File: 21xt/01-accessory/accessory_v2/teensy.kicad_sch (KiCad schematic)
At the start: 20 parts, among them Q3 BSS138, U1 DEV-16771, U2 TPS22915BYFPR

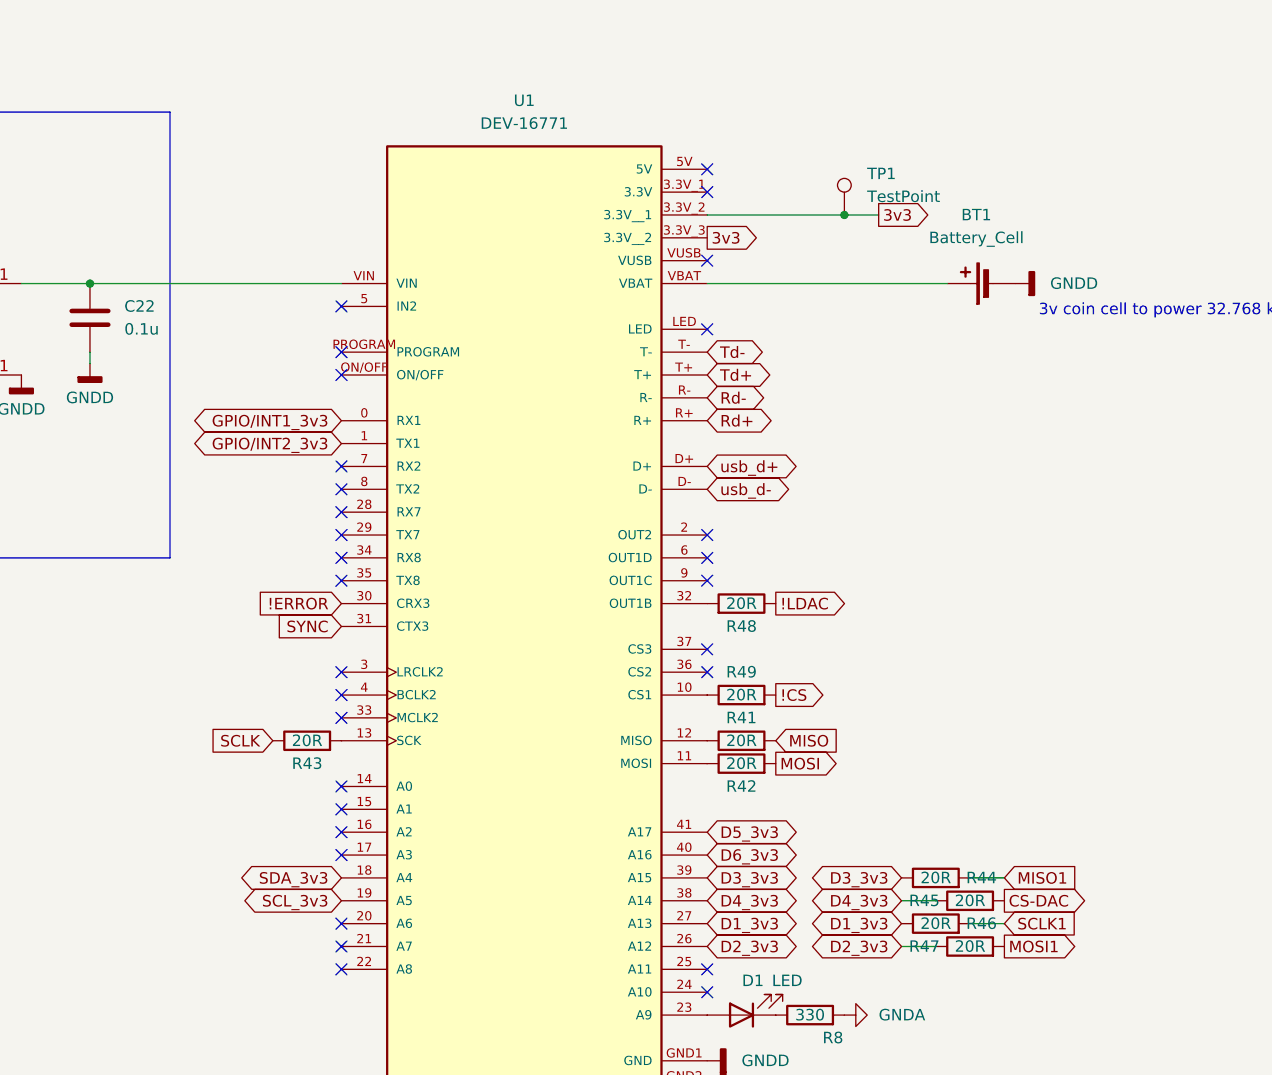
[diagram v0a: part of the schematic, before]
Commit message: laied out
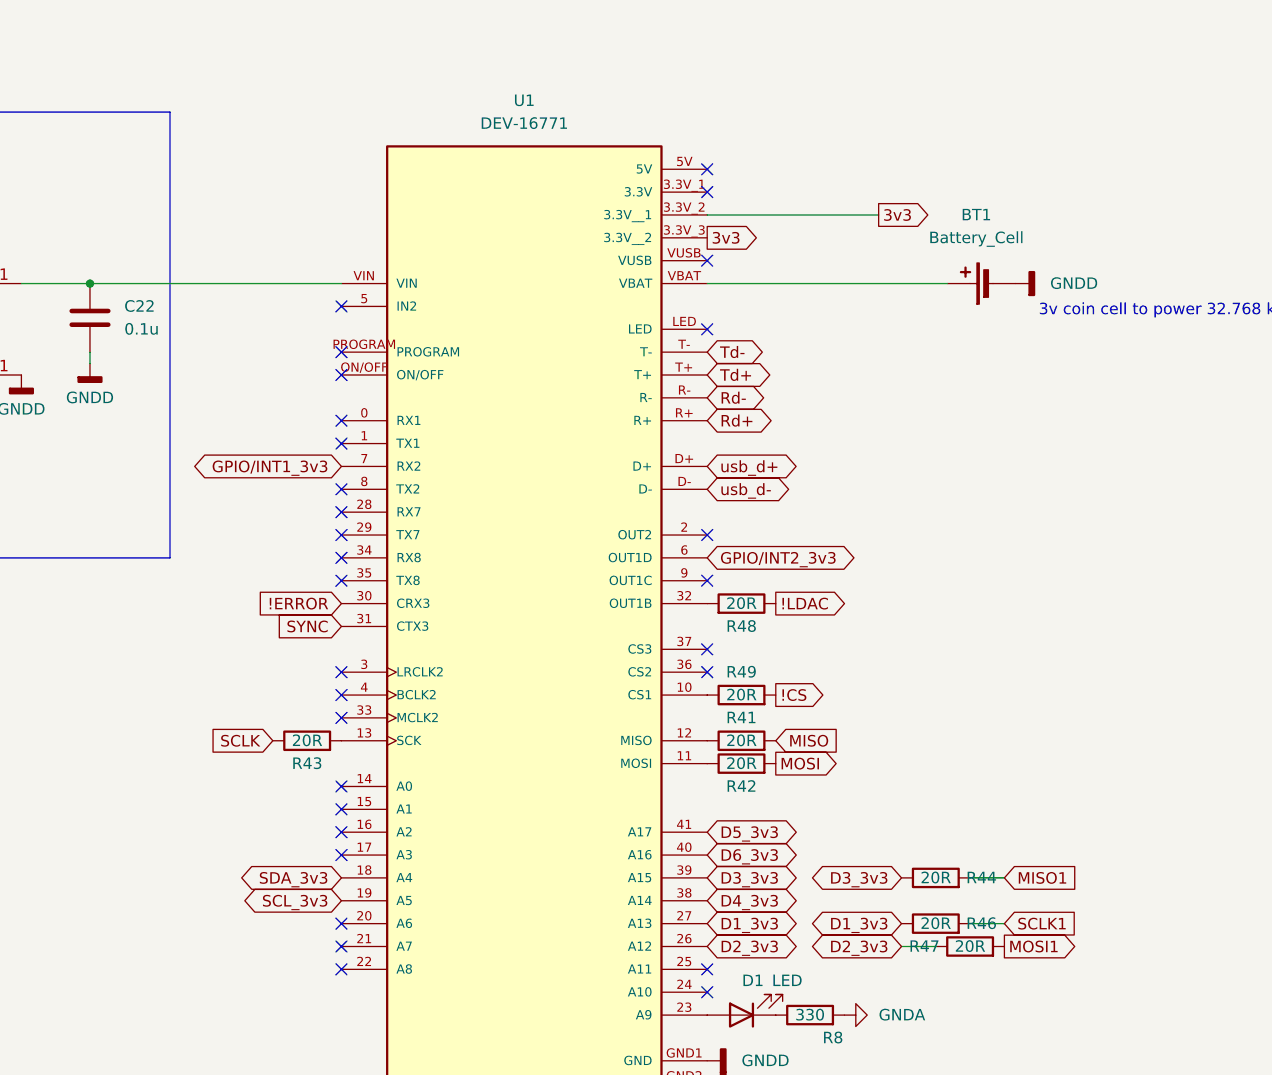
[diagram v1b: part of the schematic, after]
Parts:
- removed R45: 20R, Resistor_SMD:R_0402_1005Metric, symbol Device:R
- removed TP1: TestPoint, TestPoint:TestPoint_Pad_2.0x2.0mm, symbol Connector:TestPoint
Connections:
- net GPIO/INT1_3v3: now also U1.7 (RX2); no longer U1.0 (RX1)
- net GPIO/INT2_3v3: now also U1.6 (OUT1D); no longer U1.1 (TX1)
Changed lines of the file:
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@@
   (junction (at 34.29 69.85) (diameter 0) (color 0 0 0 0)
-  )
-  (junction (at 193.04 46.99) (diameter 0) (color 0 0 0 0)
   )
   (junction (at 109.22 54.61) (diameter 0) (color 0 0 0 0)
@@
   (no_connect (at 137.16 64.77))
   (no_connect (at 137.16 130.81))
-  (no_connect (at 177.8 85.09))
   (no_connect (at 137.16 57.15))
   (no_connect (at 137.16 118.11))
+  (no_connect (at 137.16 69.85))
   (no_connect (at 137.16 87.63))
   (no_connect (at 137.16 62.23))
-  (no_connect (at 137.16 74.93))
   (no_connect (at 137.16 102.87))
   (no_connect (at 177.8 133.35))
@@
   (no_connect (at 137.16 100.33))
   (no_connect (at 137.16 125.73))
+  (no_connect (at 137.16 72.39))
   (no_connect (at 137.16 77.47))
   (no_connect (at 177.8 59.69))
@@
     (stroke (width 0) (type default))
   )
-  (wire (pts (xy 196.85 46.99) (xy 193.04 46.99))
-    (stroke (width 0) (type default))
-  )
-  (wire (pts (xy 177.8 46.99) (xy 193.04 46.99))
+  (wire (pts (xy 177.8 46.99) (xy 196.85 46.99))
     (stroke (width 0) (type default))
   )
@@
   )
   (wire (pts (xy 58.42 50.8) (xy 58.42 52.07))
-    (stroke (width 0) (type default))
-  )
-  (wire (pts (xy 203.2 123.19) (xy 199.39 123.19))
     (stroke (width 0) (type default))
   )
@@
     )
   )
-  (global_label "CS-DAC" (shape output) (at 210.82 123.19 0) (fields_autoplaced)
-    (effects (font (size 1.27 1.27)) (justify left))
-    (property "Intersheetrefs" "${INTERSHEET_REFS}" (at 221.4857 123.19 0)
-      (effects (font (size 1.27 1.27)) (justify left) hide)
-    )
-  )
   (global_label "D4_3v3" (shape bidirectional) (at 177.8 123.19 0) (fields_autoplaced)
     (effects (font (size 1.27 1.27)) (justify left))
@@
     )
   )
-  (global_label "GPIO{slash}INT2_3v3" (shape bidirectional) (at 137.16 72.39 180) (fields_autoplaced)
-    (effects (font (size 1.27 1.27)) (justify right))
-    (property "Intersheetrefs" "${INTERSHEET_REFS}" (at 118.7911 72.39 0)
-      (effects (font (size 1.27 1.27)) (justify right) hide)
-    )
-  )
   (global_label "usb_gnd" (shape input) (at 177.8 156.21 0) (fields_autoplaced)
     (effects (font (size 1.27 1.27)) (justify left))
@@
     )
   )
-  (global_label "GPIO{slash}INT1_3v3" (shape bidirectional) (at 137.16 69.85 180) (fields_autoplaced)
-    (effects (font (size 1.27 1.27)) (justify right))
-    (property "Intersheetrefs" "${INTERSHEET_REFS}" (at 118.7911 69.85 0)
-      (effects (font (size 1.27 1.27)) (justify right) hide)
-    )
-  )
   (global_label "Td-" (shape bidirectional) (at 177.8 62.23 0) (fields_autoplaced)
     (effects (font (size 1.27 1.27)) (justify left))
@@
     )
   )
+  (global_label "GPIO{slash}INT2_3v3" (shape bidirectional) (at 177.8 85.09 0) (fields_autoplaced)
+    (effects (font (size 1.27 1.27)) (justify left))
+    (property "Intersheetrefs" "${INTERSHEET_REFS}" (at 196.1689 85.09 0)
+      (effects (font (size 1.27 1.27)) (justify left) hide)
+    )
+  )
   (global_label "Rd+" (shape bidirectional) (at 177.8 69.85 0) (fields_autoplaced)
     (effects (font (size 1.27 1.27)) (justify left))
@@
     )
   )
-  (global_label "D4_3v3" (shape bidirectional) (at 199.39 123.19 180) (fields_autoplaced)
-    (effects (font (size 1.27 1.27)) (justify right))
-    (property "Intersheetrefs" "${INTERSHEET_REFS}" (at 188.4598 123.19 0)
-      (effects (font (size 1.27 1.27)) (justify right) hide)
-    )
-  )
   (global_label "LS_EN" (shape input) (at 31.75 69.85 180) (fields_autoplaced)
     (effects (font (size 1.27 1.27)) (justify right))
@@
     (property "Intersheetrefs" "${INTERSHEET_REFS}" (at 219.6109 120.65 0)
       (effects (font (size 1.27 1.27)) (justify left) hide)
+    )
+  )
+  (global_label "GPIO{slash}INT1_3v3" (shape bidirectional) (at 137.16 74.93 180) (fields_autoplaced)
+    (effects (font (size 1.27 1.27)) (justify right))
+    (property "Intersheetrefs" "${INTERSHEET_REFS}" (at 118.7911 74.93 0)
+      (effects (font (size 1.27 1.27)) (justify right) hide)
     )
   )
@@
         (path "/5dacc41e-ffff-47d3-9300-200c6018c603/632615cf-95a2-44a3-ae6d-1166f38afe7f"
           (reference "R19") (unit 1)
-        )
-      )
-    )
-  )
-  (symbol (lib_id "Device:R") (at 207.01 123.19 90) (unit 1)
-    (in_bom yes) (on_board yes) (dnp no)
-    (property "Reference" "R45" (at 201.93 123.19 90)
-      (effects (font (size 1.27 1.27)))
-    )
-    (property "Value" "20R" (at 207.01 123.19 90)
-      (effects (font (size 1.27 1.27)))
-    )
-    (property "Footprint" "Resistor_SMD:R_0402_1005Metric" (at 207.01 124.968 90)
-      (effects (font (size 1.27 1.27)) hide)
-    )
-    (property "Datasheet" "~" (at 207.01 123.19 0)
-      (effects (font (size 1.27 1.27)) hide)
-    )
-    (pin "1")
-    (pin "2")
-    (instances
-      (project "accessory_v2"
-        (path "/5dacc41e-ffff-47d3-9300-200c6018c603/632615cf-95a2-44a3-ae6d-1166f38afe7f"
-          (reference "R45") (unit 1)
         )
       )
@@
         )
       )
-    )
-  )
-  (symbol (lib_id "Connector:TestPoint") (at 193.04 46.99 0) (unit 1)
-    (in_bom yes) (on_board yes) (dnp no) (fields_autoplaced)
-    (property "Reference" "TP1" (at 195.58 42.418 0)
-      (effects (font (size 1.27 1.27)) (justify left))
-    )
-    (property "Value" "TestPoint" (at 195.58 44.958 0)
-      (effects (font (size 1.27 1.27)) (justify left))
-    )
-    (property "Footprint" "TestPoint:TestPoint_Pad_2.0x2.0mm" (at 198.12 46.99 0)
-      (effects (font (size 1.27 1.27)) hide)
-    )
-    (property "Datasheet" "~" (at 198.12 46.99 0)
-      (effects (font (size 1.27 1.27)) hide)
-    )
-    (pin "1")
-    (instances
-      (project "accessory_v2"
-        (path "/5dacc41e-ffff-47d3-9300-200c6018c603/632615cf-95a2-44a3-ae6d-1166f38afe7f"
-          (reference "TP1") (unit 1)
-        )
-      )
